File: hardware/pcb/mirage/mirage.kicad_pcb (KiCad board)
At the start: 2 copper layers, 36.6 x 68.3 mm, 4 parts, among them U1 Adafruit ST7735R, U2 ESP32-S3-WROOM-1-N8

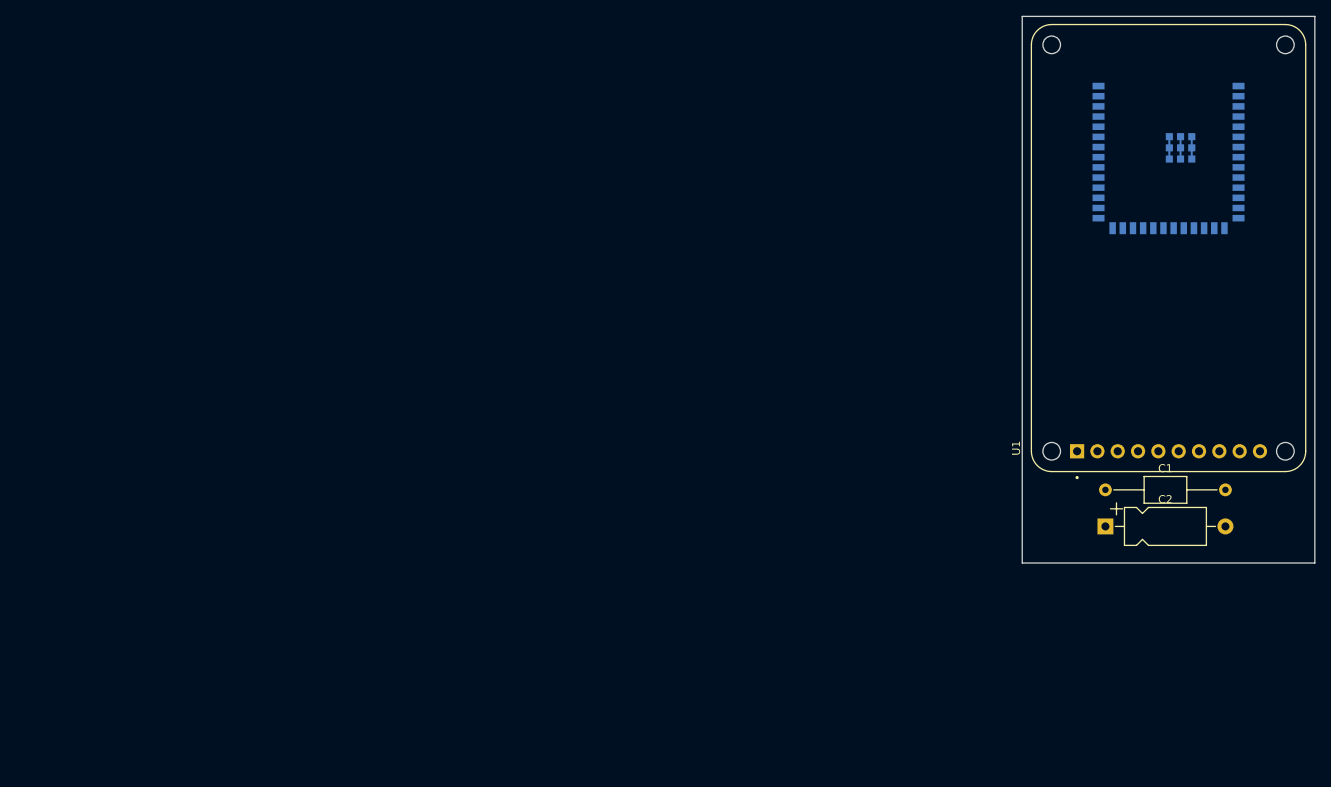
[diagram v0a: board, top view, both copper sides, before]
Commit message: feat: temporary pcb/schematic work
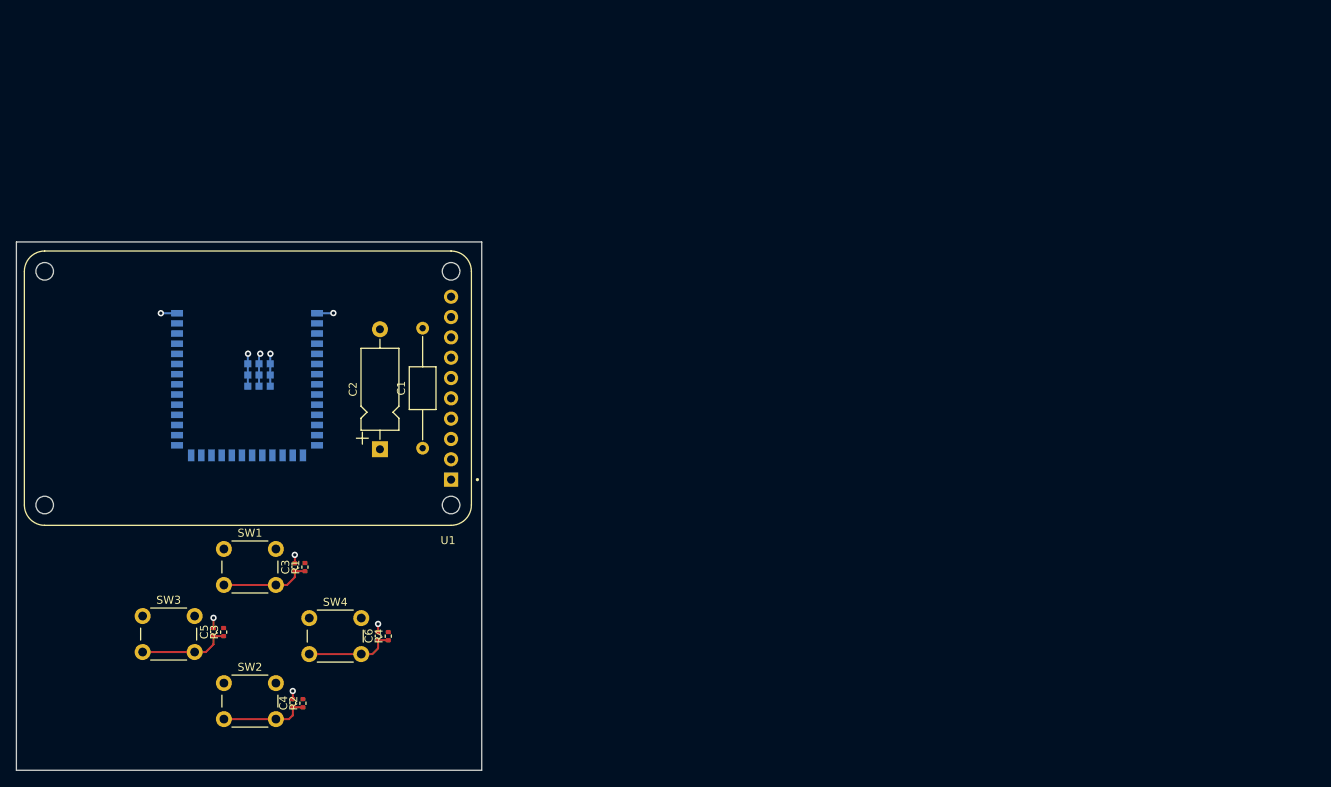
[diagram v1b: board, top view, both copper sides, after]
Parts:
- added C3: 100 nf, Capacitor_SMD:C_0402_1005Metric, F.Cu at (63.8, 104.4)
- added C4: 100 nf, Capacitor_SMD:C_0402_1005Metric, F.Cu at (63.5, 121.4)
- added C5: 100 nf, Capacitor_SMD:C_0402_1005Metric, F.Cu at (53.6, 112.5)
- added C6: 100 nf, Capacitor_SMD:C_0402_1005Metric, F.Cu at (74.2, 113.0)
- added R1: 100K, Resistor_SMD:R_0402_1005Metric, F.Cu at (65.0, 104.4)
- added R2: 100K, Resistor_SMD:R_0402_1005Metric, F.Cu at (64.8, 121.4)
- added R3: 100K, Resistor_SMD:R_0402_1005Metric, F.Cu at (54.9, 112.5)
- added R4: 100K, Resistor_SMD:R_0402_1005Metric, F.Cu at (75.4, 113.0)
- added SW1: UP, Button_Switch_THT:SW_PUSH_6mm, F.Cu at (54.9, 102.1)
- added SW2: DOWN, Button_Switch_THT:SW_PUSH_6mm, F.Cu at (54.9, 118.9)
- added SW3: LEFT, Button_Switch_THT:SW_PUSH_6mm, F.Cu at (44.7, 110.5)
- added SW4: RIGHT, Button_Switch_THT:SW_PUSH_6mm, F.Cu at (65.6, 110.8)
- moved U2 118.6 mm to (57.8, 77.9)
- moved U1 116.4 mm to (57.9, 82.0), turned to 180 degrees
- moved C2 91.2 mm to (74.4, 89.7), turned to 90 degrees
- moved C1 85.5 mm to (79.7, 89.5), turned to 90 degrees
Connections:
- U2 pad 33: unconnected-(U2-IO40-Pad33) -> /TFT_D/C
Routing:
- net GND: track 8.40 -> 20.7 mm, vias 0 -> 9
- net /SW_LEFT: track 0.00 -> 11.6 mm
- net /SW_UP: track 0.00 -> 11.3 mm
- net /SW_RIGHT: track 0.00 -> 11.3 mm
- net /SW_DOWN: track 0.00 -> 11.2 mm
- added copper zone on In1.Cu, net GND
- added copper zone on In2.Cu, net GND
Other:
- board size 36.6 x 68.3 mm -> 58.2 x 66 mm
- copper layers 2 -> 4

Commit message: fix: changed ST7735 pins to ESP32
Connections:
- U2 pad 33: /TFT_D/C -> unconnected-(U2-IO40-Pad33)
- U2 pad 34: /TFT_RST -> unconnected-(U2-IO41-Pad34)
- U2 pad 35: /TFT_CS -> unconnected-(U2-IO42-Pad35)
- U2 pad 38: unconnected-(U2-IO2-Pad38) -> /TFT_D/C
- U2 pad 4: unconnected-(U2-IO4-Pad4) -> /TFT_RST
- U2 pad 5: unconnected-(U2-IO5-Pad5) -> /TFT_CS
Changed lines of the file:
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@@
   (net 9 "/TFT_RST")
   (net 10 "unconnected-(U2-EN-Pad3)")
-  (net 11 "unconnected-(U2-IO4-Pad4)")
-  (net 12 "unconnected-(U2-IO5-Pad5)")
+  (net 11 "unconnected-(U2-IO40-Pad33)")
+  (net 12 "unconnected-(U2-IO41-Pad34)")
   (net 13 "unconnected-(U2-IO6-Pad6)")
   (net 14 "unconnected-(U2-IO7-Pad7)")
@@
   (net 37 "unconnected-(U2-RXD0-Pad36)")
   (net 38 "unconnected-(U2-TXD0-Pad37)")
-  (net 39 "unconnected-(U2-IO2-Pad38)")
+  (net 39 "unconnected-(U2-IO42-Pad35)")
   (net 40 "unconnected-(U2-IO1-Pad39)")
   (net 41 "/SW_UP")
@@
       (net 10 "unconnected-(U2-EN-Pad3)") (pinfunction "EN") (pintype "input"))
     (pad "4" smd rect (at -8.75 1.45 180) (size 1.4986 0.8128) (layers "B.Cu" "B.Paste" "B.Mask")
-      (net 11 "unconnected-(U2-IO4-Pad4)") (pinfunction "IO4") (pintype "bidirectional"))
+      (net 9 "/TFT_RST") (pinfunction "IO4") (pintype "bidirectional"))
     (pad "5" smd rect (at -8.75 0.18 180) (size 1.4986 0.8128) (layers "B.Cu" "B.Paste" "B.Mask")
-      (net 12 "unconnected-(U2-IO5-Pad5)") (pinfunction "IO5") (pintype "bidirectional"))
+      (net 6 "/TFT_CS") (pinfunction "IO5") (pintype "bidirectional"))
     (pad "6" smd rect (at -8.75 -1.09 180) (size 1.4986 0.8128) (layers "B.Cu" "B.Paste" "B.Mask")
       (net 13 "unconnected-(U2-IO6-Pad6)") (pinfunction "IO6") (pintype "bidirectional"))
@@
       (net 36 "unconnected-(U2-IO39-Pad32)") (pinfunction "IO39") (pintype "bidirectional"))
     (pad "33" smd rect (at 8.75 -3.63 180) (size 1.4986 0.8128) (layers "B.Cu" "B.Paste" "B.Mask")
-      (net 8 "/TFT_D{slash}C") (pinfunction "IO40") (pintype "bidirectional"))
+      (net 11 "unconnected-(U2-IO40-Pad33)") (pinfunction "IO40") (pintype "bidirectional"))
     (pad "34" smd rect (at 8.75 -2.36 180) (size 1.4986 0.8128) (layers "B.Cu" "B.Paste" "B.Mask")
-      (net 9 "/TFT_RST") (pinfunction "IO41") (pintype "bidirectional"))
+      (net 12 "unconnected-(U2-IO41-Pad34)") (pinfunction "IO41") (pintype "bidirectional"))
     (pad "35" smd rect (at 8.75 -1.09 180) (size 1.4986 0.8128) (layers "B.Cu" "B.Paste" "B.Mask")
-      (net 6 "/TFT_CS") (pinfunction "IO42") (pintype "bidirectional"))
+      (net 39 "unconnected-(U2-IO42-Pad35)") (pinfunction "IO42") (pintype "bidirectional"))
     (pad "36" smd rect (at 8.75 0.18 180) (size 1.4986 0.8128) (layers "B.Cu" "B.Paste" "B.Mask")
       (net 37 "unconnected-(U2-RXD0-Pad36)") (pinfunction "RXD0") (pintype "bidirectional"))
@@
       (net 38 "unconnected-(U2-TXD0-Pad37)") (pinfunction "TXD0") (pintype "bidirectional"))
     (pad "38" smd rect (at 8.75 2.72 180) (size 1.4986 0.8128) (layers "B.Cu" "B.Paste" "B.Mask")
-      (net 39 "unconnected-(U2-IO2-Pad38)") (pinfunction "IO2") (pintype "bidirectional"))
+      (net 8 "/TFT_D{slash}C") (pinfunction "IO2") (pintype "bidirectional"))
     (pad "39" smd rect (at 8.75 3.99 180) (size 1.4986 0.8128) (layers "B.Cu" "B.Paste" "B.Mask")
       (net 40 "unconnected-(U2-IO1-Pad39)") (pinfunction "IO1") (pintype "bidirectional"))

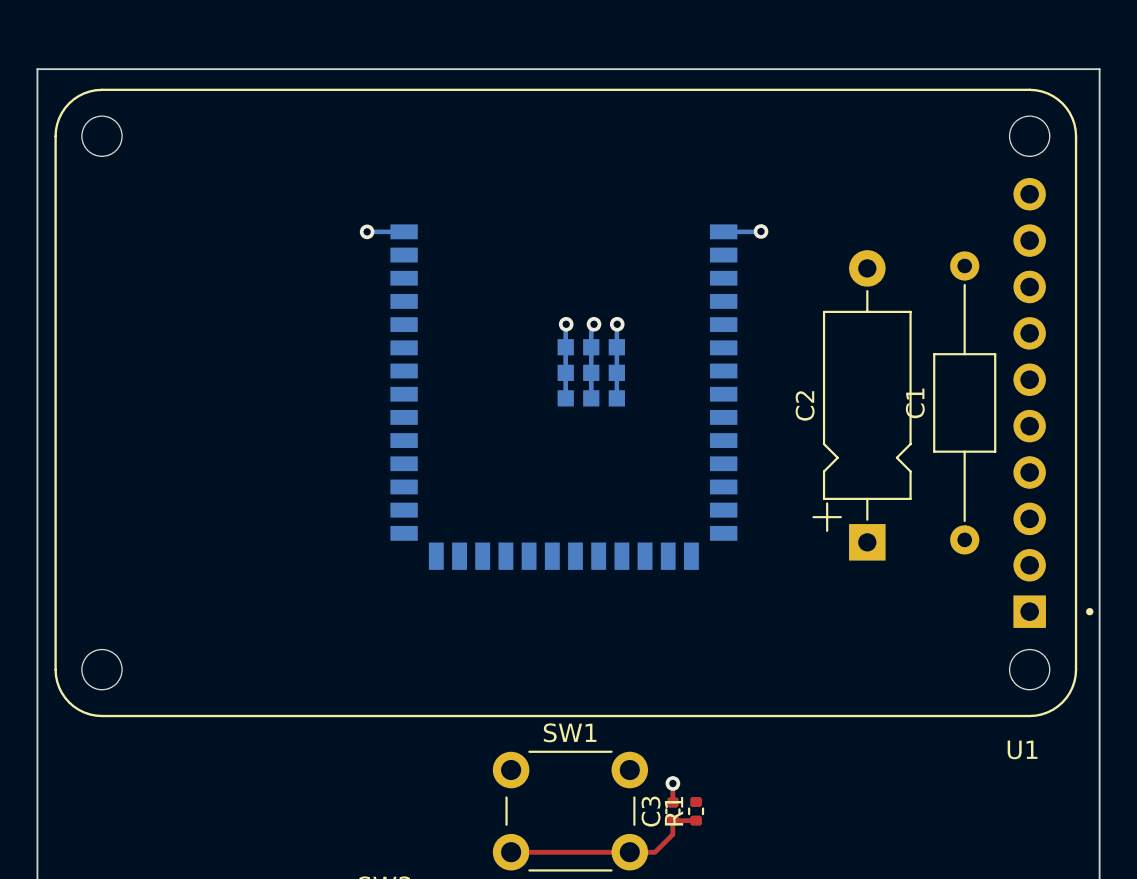
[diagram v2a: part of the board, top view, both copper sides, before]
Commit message: feat: added footprints, schematics, and models
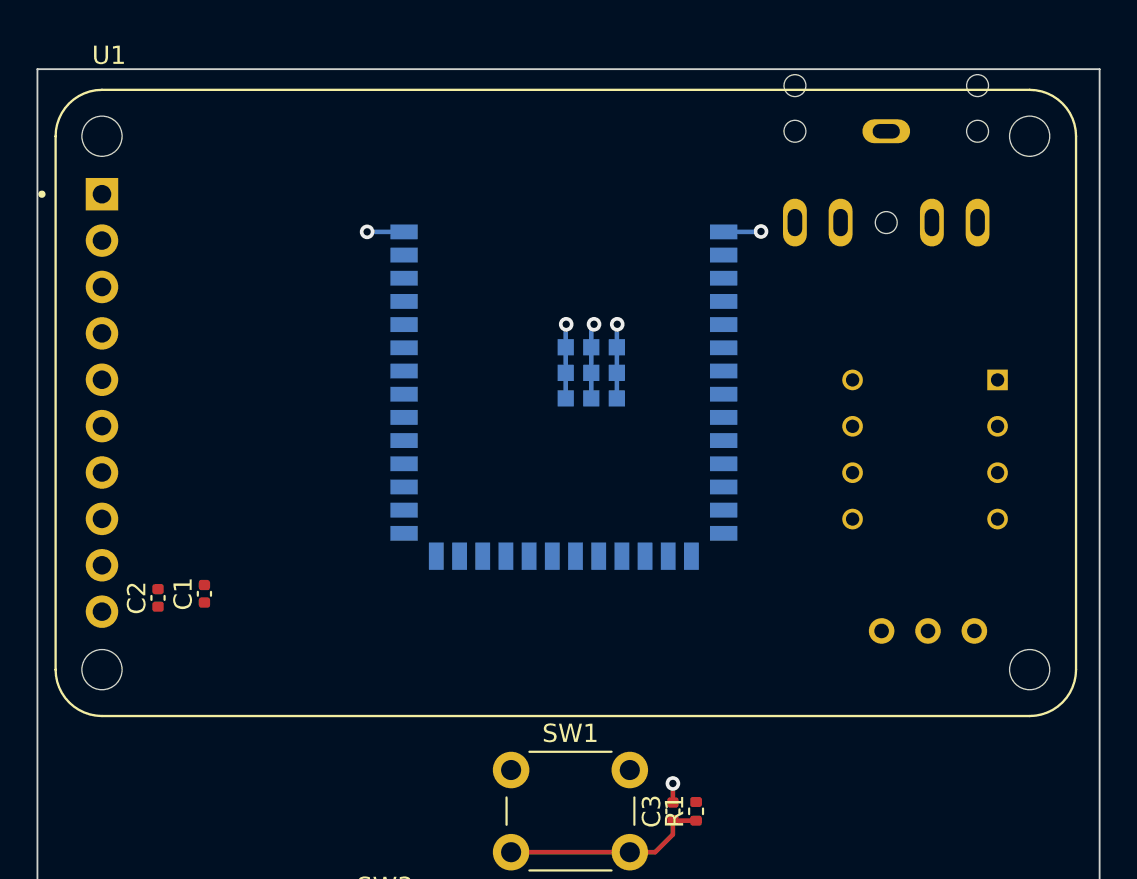
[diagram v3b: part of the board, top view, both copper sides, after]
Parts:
- added IC1: TLV5618AIP, footprints:ti_TLV5618AIP, B.Cu at (77.6, 84.6)
- added IC2: LM4041CILPR, footprints:ti_LM4041CILPR, B.Cu at (77.7, 94.5)
- added J1: SJ1-3525N, footprints:PJ-307, B.Cu at (75.4, 67.2)
- C1: footprint Capacitor_THT:C_Axial_L5.1mm_D3.1mm_P15.00mm_Horizontal -> Capacitor_SMD:C_0402_1005Metric
- C2: footprint Capacitor_THT:CP_Axial_L10.0mm_D4.5mm_P15.00mm_Horizontal -> Capacitor_SMD:C_0402_1005Metric
- moved C1 41.7 mm to (38.1, 92.5)
- moved C2 39.0 mm to (35.6, 92.7)
- turned U1 to 0 degrees
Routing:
- net /TFT_MISO: track 0.00 -> 0.54 mm
- removed copper zone on In1.Cu, net GND
- removed copper zone on In2.Cu, net GND
